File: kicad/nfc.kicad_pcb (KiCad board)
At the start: 2 copper layers, 89 x 51 mm, 9 parts, among them Con1 trace, U1 NT3H2111W0FHKH

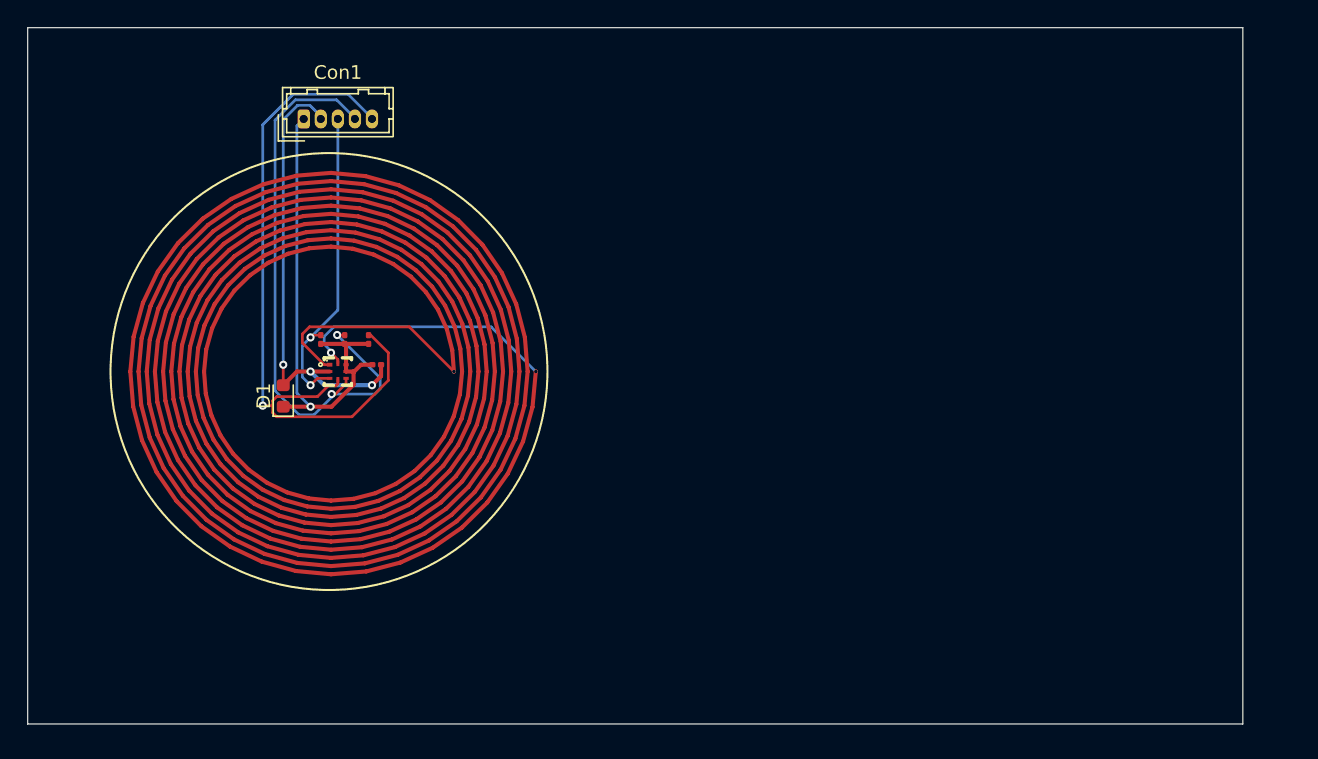
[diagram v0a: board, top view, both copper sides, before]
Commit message: done
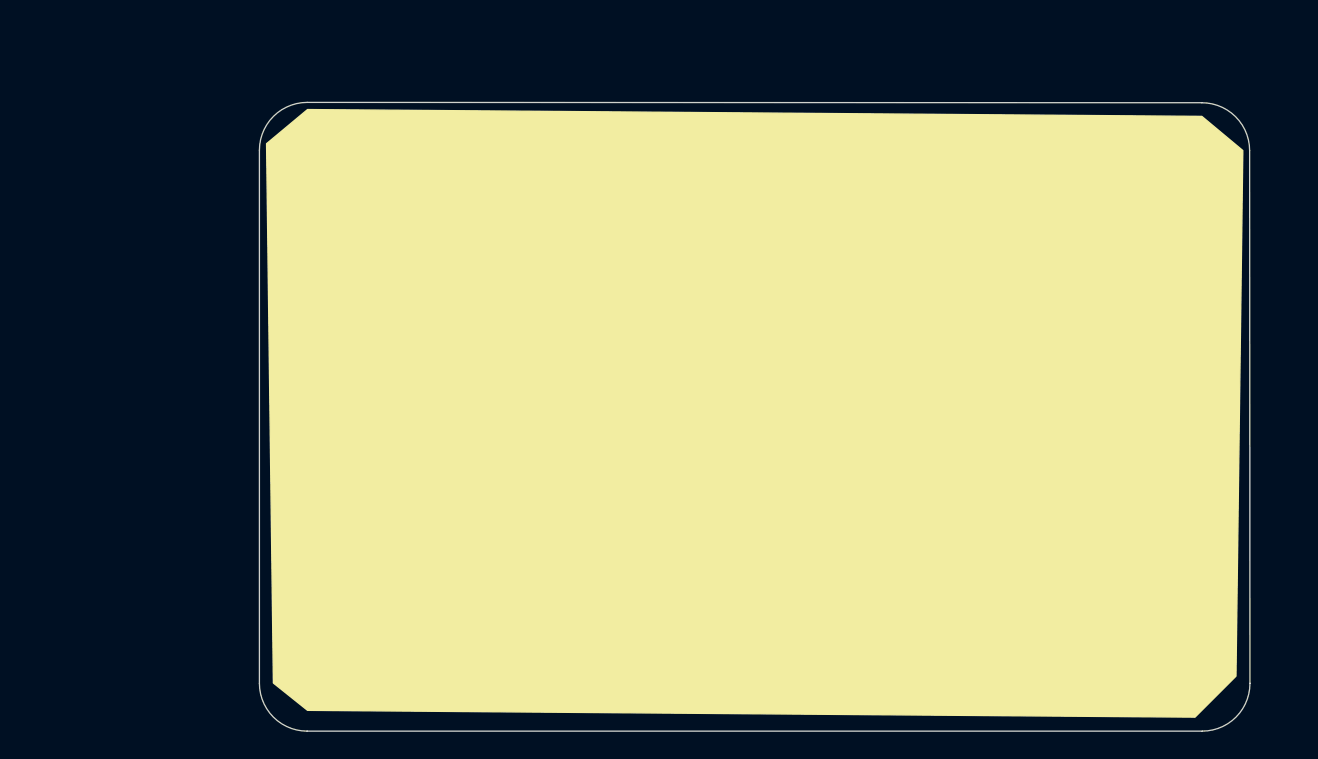
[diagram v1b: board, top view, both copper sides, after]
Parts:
- removed the G*** at (1378.0, 597.5)
- added G***: LOGO, archbtw:wifi, B.Cu at (1343.5, 592.5)
- added G***: LOGO, archbtw:octocat, B.Cu at (1369.5, 579.0)
- added G***: LOGO, archbtw:hc, B.Cu at (1343.4, 608.0)
- added G***: LOGO, archbtw:qrfin, B.Cu at (1386.5, 580.5)
- Cap1: value 150-220nf -> 180 nf; footprint Capacitor_SMD:C_0201_0603Metric -> Capacitor_SMD:C_0402_1005Metric
- R1, R2, R3: footprint Resistor_SMD:R_0201_0603Metric -> Resistor_SMD:R_0402_1005Metric
- moved Cap1 14.2 mm to (1347.3, 595.8)
- moved Con1 14.2 mm to (1342.0, 577.8)
- moved D1 14.2 mm to (1340.5, 598.1)
- moved L1 14.2 mm to (1343.8, 581.3)
- moved R1 14.2 mm to (1343.2, 593.9)
- moved R2 14.2 mm to (1345.0, 593.9)
- moved R3 14.2 mm to (1346.8, 593.9)
- moved U1 14.2 mm to (1344.5, 596.3)
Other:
- board size 89 x 51 mm -> 72.6 x 46.1 mm
- board text added: "I use arch , Btw"
- board text removed: "I use arch , btw"

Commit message: ok kinda done gonna tune right now again
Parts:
- Cap1: footprint Capacitor_SMD:C_0402_1005Metric -> Capacitor_SMD:C_0603_1608Metric
- Con1: value trace -> Conn_01x05_Pin
- L1: footprint antenna:ftprnt -> footprint:ftprnt
- R1, R2, R3: footprint Resistor_SMD:R_0402_1005Metric -> Resistor_SMD:R_0603_1608Metric
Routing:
- net +2V8: track 36.2 -> 37.7 mm
